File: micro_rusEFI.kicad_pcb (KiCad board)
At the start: 2 copper layers, 80.6 x 93.7 mm, 167 parts, among them J1 USB_B_Micro, J19 Conn_01x06, J2 Conn_02x05_Odd_Even, J4 Conn_02x05_Counter_Clockwise, J7 TC2030, Q1 IPD30N06S2L-23, SW1 SW_Push, SW2 SW_Push, SW3 SW_Push, SW4 SW_Push, U1 STM32F427VGT6, U3 molex_48pin_MRE, U35 MCP6004, U36 MCP6004, U46 MCP6004, U5 LM1117-3.3, U8 MCP6004, X1 8MHz 20pF, Y2 32768 Hz

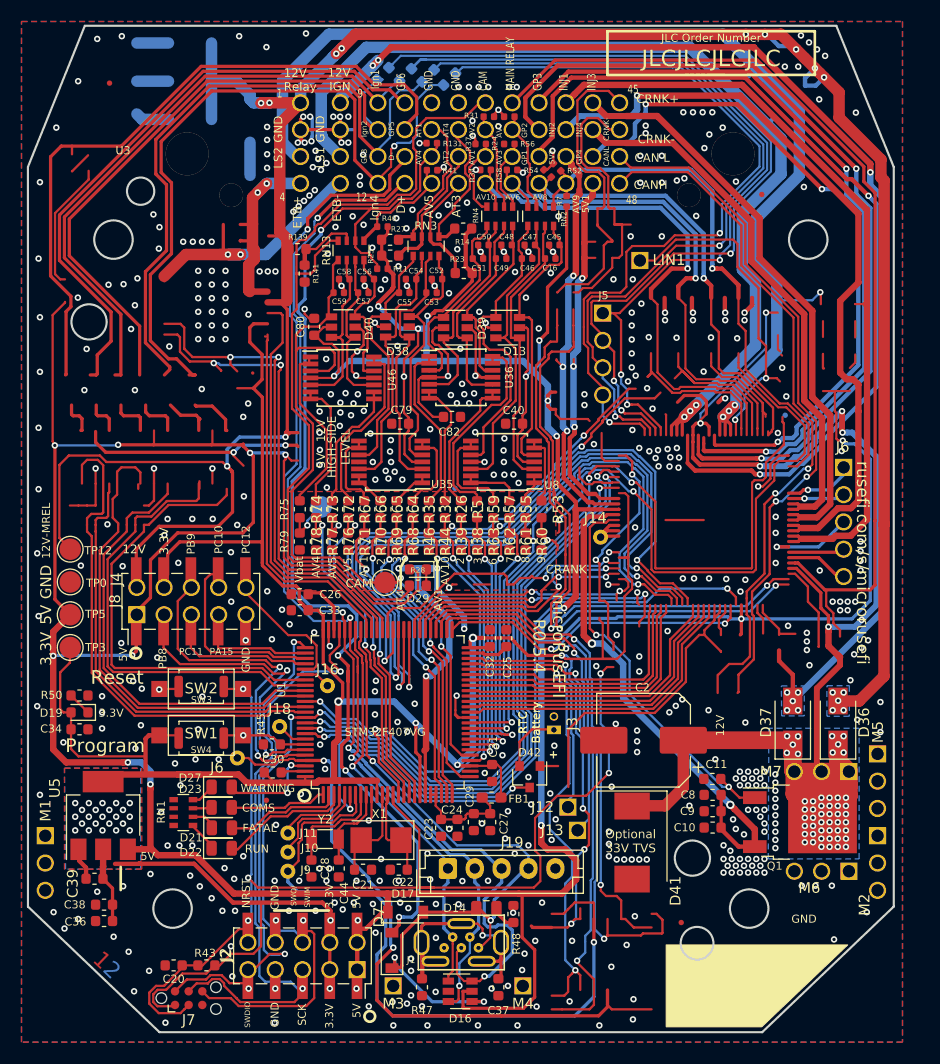
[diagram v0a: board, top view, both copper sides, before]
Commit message: First commit
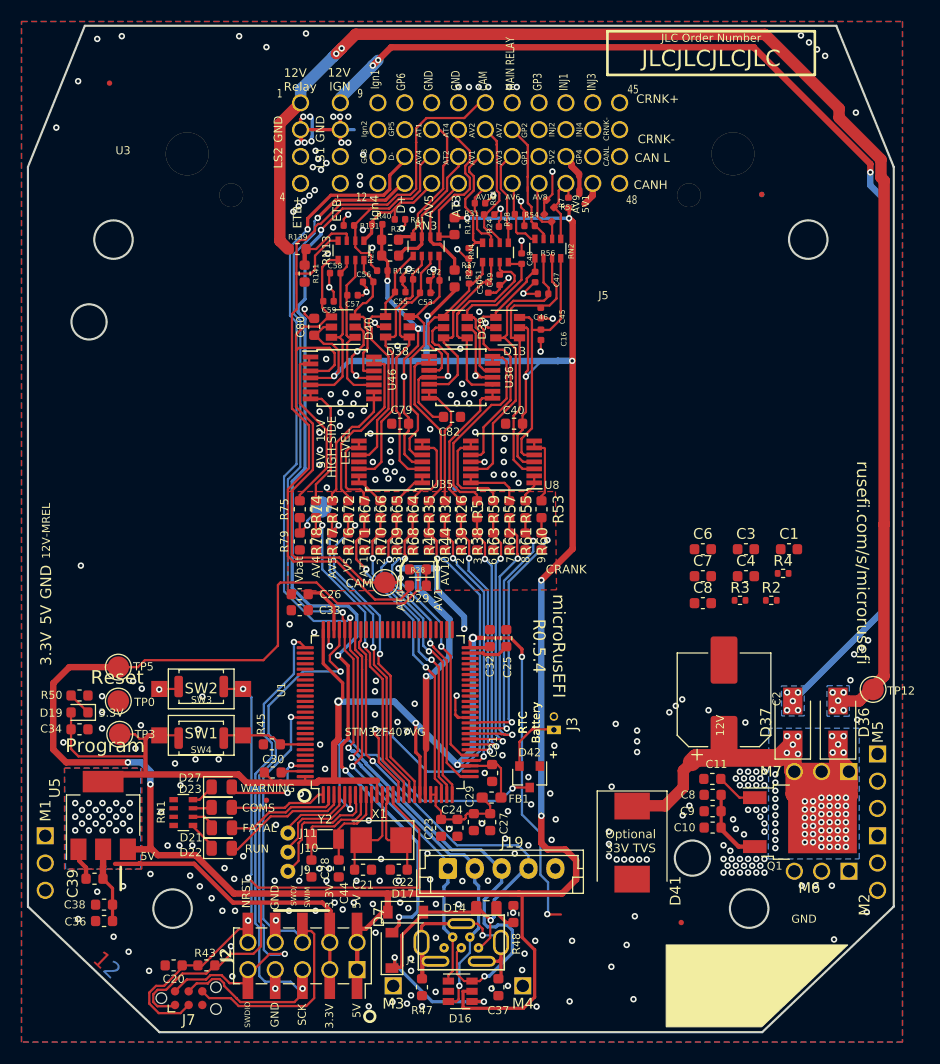
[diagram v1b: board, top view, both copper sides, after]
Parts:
- removed J4: Conn_02x05_Counter_Clockwise, Connector_PinHeader_2.54mm:PinHeader_2x05_P2.54mm_Vertical_SMD
- removed R21, R33, R80, R81: 0R, Resistor_SMD:R_0603_1608Metric
- added C1: 4.7u, Capacitor_SMD:C_0603_1608Metric, F.Cu at (91.4, 71.1)
- added C3: 1u, Capacitor_SMD:C_0603_1608Metric, F.Cu at (87.4, 71.1)
- added C4: 10n, Capacitor_SMD:C_0603_1608Metric, F.Cu at (87.4, 73.6)
- added C6: 270p, Capacitor_SMD:C_0603_1608Metric, F.Cu at (83.4, 71.1)
- added C7: 10u, Capacitor_SMD:C_0603_1608Metric, F.Cu at (83.4, 73.6)
- added C8: 10u, Capacitor_SMD:C_0603_1608Metric, F.Cu at (83.4, 76.1)
- added R2: 10k, Resistor_SMD:R_0402_1005Metric, F.Cu at (89.8, 75.9)
- added R3: 12k, Resistor_SMD:R_0402_1005Metric, F.Cu at (86.9, 75.9)
- added R4: 68k, Resistor_SMD:R_0402_1005Metric, F.Cu at (90.9, 73.4)
- moved TP12 75.9 mm to (99.3, 84.2)
- moved FID5 20.7 mm to (88.9, 38.1)
- moved TP0 12.0 mm to (29.0, 85.3)
- moved R131 10.9 mm to (50.5, 41.0)
- moved R56 10.3 mm to (67.3, 41.0)
- moved R37 10.2 mm to (61.6, 43.6), turned to -90 degrees
- moved TP3 9.30 mm to (29.1, 88.3)
- moved R31 9.11 mm to (63.5, 40.0)
- moved C16 8.46 mm to (68.3, 51.2), turned to -90 degrees
- moved C2 8.38 mm to (85.4, 85.1), turned to 90 degrees
- moved R24 7.70 mm to (64.9, 41.1)
- moved TP5 6.62 mm to (29.0, 82.1)
- moved R41 5.47 mm to (55.2, 40.4)
- moved C45 5.14 mm to (68.3, 49.1), turned to -90 degrees
- moved C46 4.72 mm to (68.6, 47.3)
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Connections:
- C2 pad 1: /12V_SAFE -> Net-(2.2u1-Pad2)
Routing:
- net (no net): track 434.4 -> 0.00 mm, vias 15 -> 0
- net /5V: track 467.3 -> 320.7 mm, vias 25 -> 14
- net unconnected-(U3-Pad3): track 106.9 -> 0.00 mm, vias 4 -> 0
- net /VDD: track 298.4 -> 193.7 mm, vias 33 -> 29
- net /12V_MREL: track 229.9 -> 131.6 mm, vias 16 -> 7
- net unconnected-(U3-Pad7): track 94.2 -> 0.00 mm, vias 3 -> 0
- net /MAIN_RELAY: track 92.0 -> 0.00 mm
- net /12V_SAFE: track 140.7 -> 49.0 mm, vias 57 -> 51
- net unconnected-(U3-Pad35): track 83.1 -> 0.00 mm, vias 2 -> 0
- net Net-(R33-Pad2): track 81.9 -> 0.00 mm, vias 3 -> 0
- net unconnected-(U3-Pad34): track 80.5 -> 0.00 mm, vias 2 -> 0
- net Net-(R21-Pad2): track 78.8 -> 0.00 mm, vias 3 -> 0
- net Net-(R80-Pad2): track 75.7 -> 0.00 mm, vias 2 -> 0
- net Net-(R81-Pad2): track 74.9 -> 0.00 mm, vias 2 -> 0
- net unconnected-(U3-Pad37): track 72.8 -> 0.10 mm
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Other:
- outline, holes or cut-outs redrawn

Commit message: did stuff
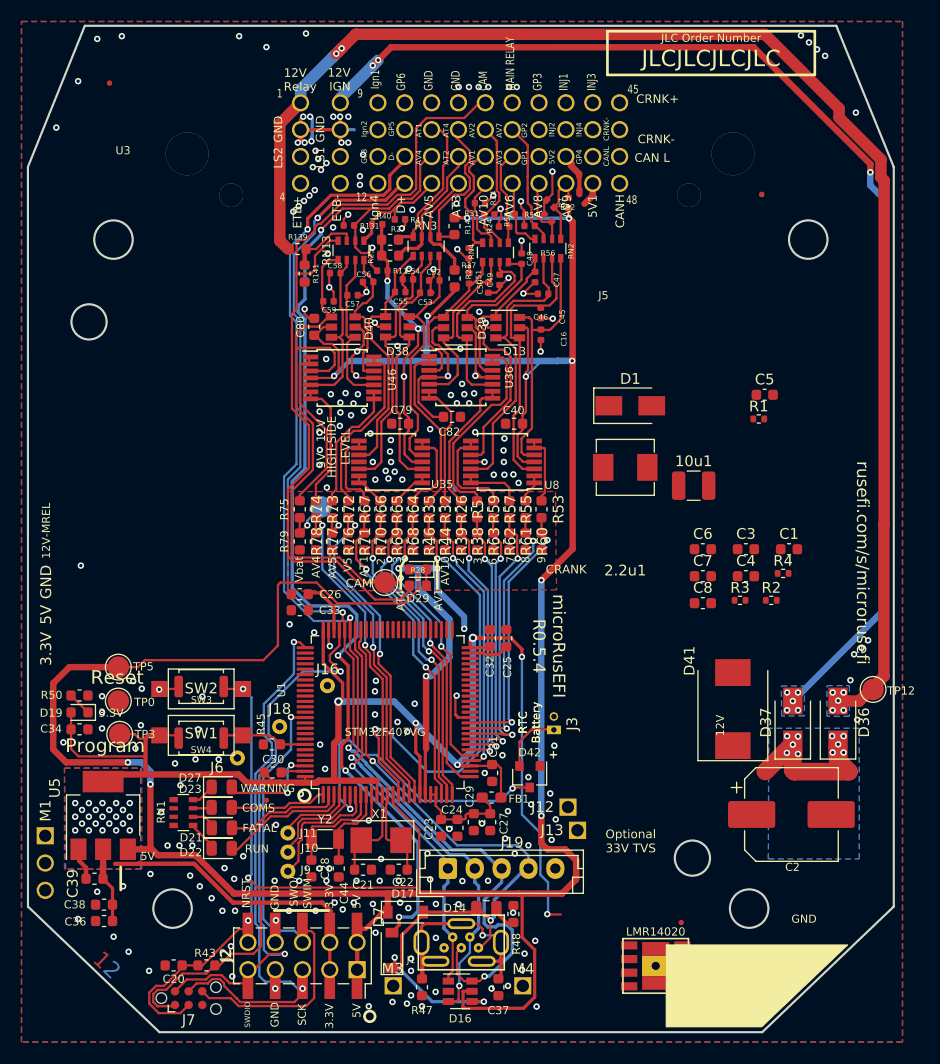
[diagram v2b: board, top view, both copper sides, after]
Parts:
- removed C10: 100nF, Capacitor_SMD:C_0603_1608Metric
- removed C11: 4.7nF, Capacitor_SMD:C_0603_1608Metric
- removed the C8 at (84.3, 94.0)
- removed C9: 10uF, Capacitor_SMD:C_0603_1608Metric
- removed Q1: IPD30N06S2L-23, Package_TO_SOT_SMD:TO-252-2
- added 10u1: L_Small, Inductor_SMD:L_1210_3225Metric, F.Cu at (82.6, 65.2)
- added 2.2u1: INDUCTOR, Simon:MWSA0503, F.Cu at (76.2, 63.5)
- added C5: 100n, Capacitor_SMD:C_0603_1608Metric, F.Cu at (89.2, 56.7)
- added D1: D_Schottky, Diode_SMD:D_SMA, F.Cu at (76.7, 57.8)
- added R1: 1, Resistor_SMD:R_0402_1005Metric, F.Cu at (88.6, 59.0)
- added U2: LMR14020, Simon:SOIC8-DFN, F.Cu at (79.0, 109.9)
- U3: footprint rusefi_lib:Molex_48_MRE -> rusefi_lib:Molex_48_BCM
- moved D41 15.6 mm to (86.2, 86.0), turned to 90 degrees
- moved C2 12.4 mm to (91.7, 95.8), turned to 0 degrees
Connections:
- C2 pad 1: Net-(2.2u1-Pad2) -> /12V_SAFE
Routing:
- net /12V_SAFE: track 49.0 -> 14.2 mm, vias 51 -> 10
- net /TLE8888-1QK/V6V: track 7.01 -> 0.00 mm
- net /TLE8888-1QK/V6GATE: track 3.89 -> 0.00 mm
- net GND: vias 314 -> 228
